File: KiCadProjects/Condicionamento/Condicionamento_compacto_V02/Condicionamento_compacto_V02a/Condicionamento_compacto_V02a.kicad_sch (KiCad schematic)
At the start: 28 parts, among them J2 Canais, J3 Entrada, J6 In_1 select, J7 In_2 select, U1-buffer1 AD828AN, U2-gain1 AD828AN, U3-Cond-DIP1 AD828AN, U4-Cond-SMD1 AD8056ARZ, U4-DigPot2 X9c10x, U5-DigPot1 X9c10x, U5-buffer1 AD8056ARZ, U6-gain1 AD8056ARZ

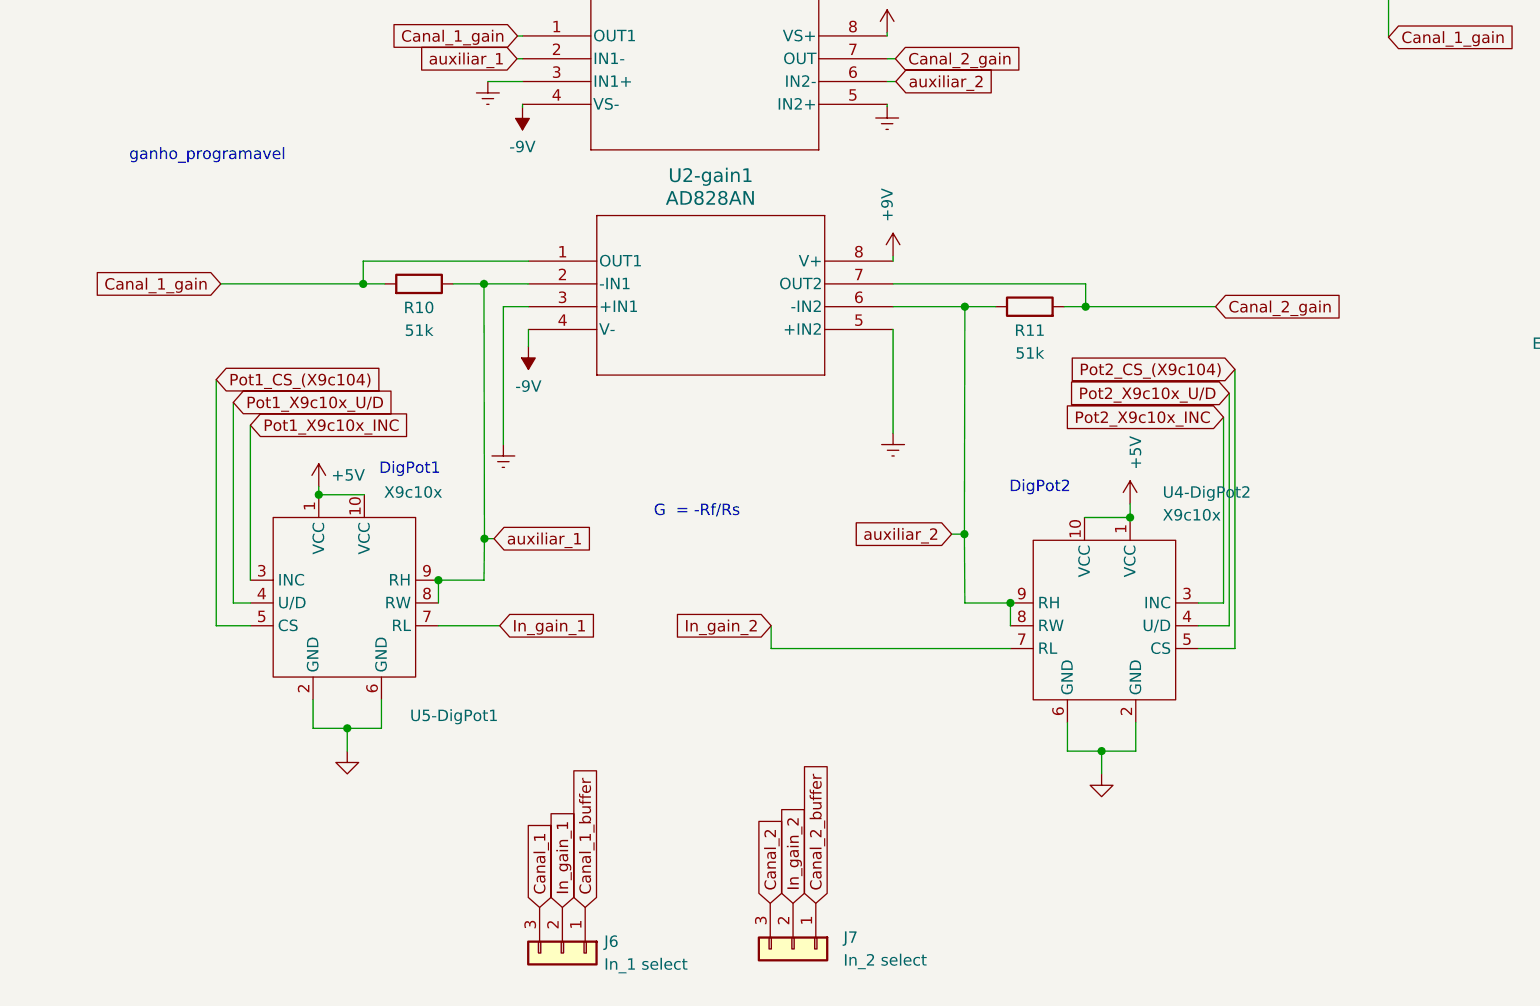
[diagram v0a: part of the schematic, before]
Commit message: tmp
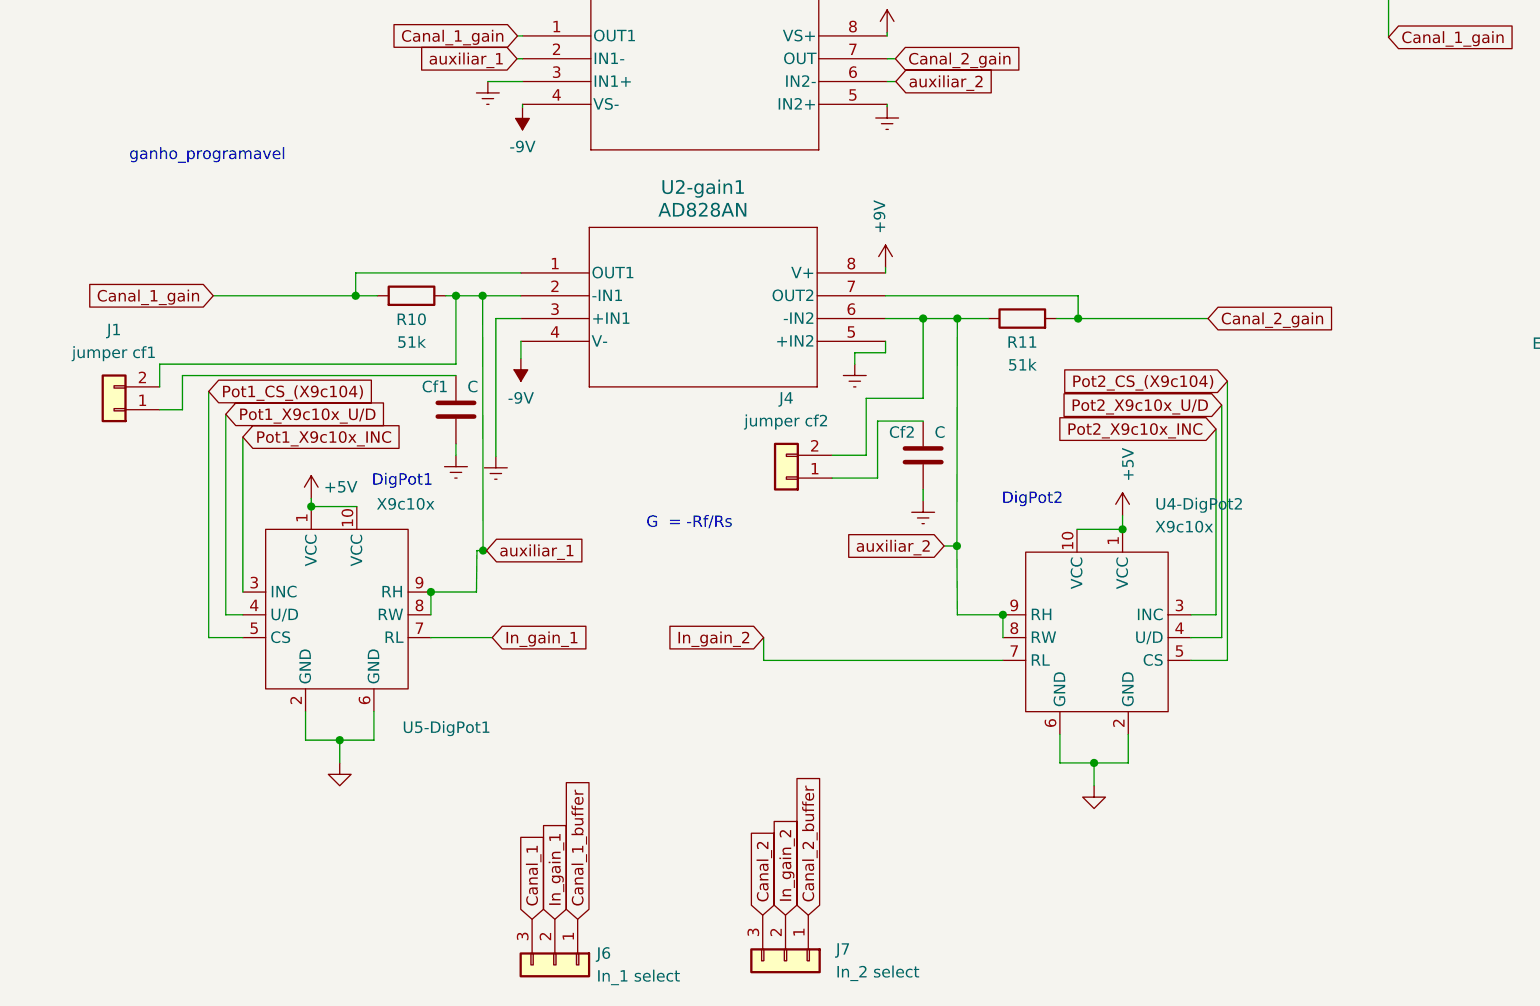
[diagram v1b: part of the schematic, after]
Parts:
- added Cf1, Cf2: C, symbol Device:C
- added J1: jumper cf1, symbol Connector_Generic:Conn_01x02
- added J4: jumper cf2, symbol Connector_Generic:Conn_01x02
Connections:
- net Earth: now also Cf1.2, Cf2.2
- net auxiliar_1: now also J1.2 (Pin_2)
- net auxiliar_2: now also J4.2 (Pin_2)
- new net: Cf1.1, J1.1 (Pin_1)
- new net: Cf2.1, J4.1 (Pin_1)
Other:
- moved on the sheet: J6, J7, R10, R11, U2-gain1, U4-DigPot2, U5-DigPot1
